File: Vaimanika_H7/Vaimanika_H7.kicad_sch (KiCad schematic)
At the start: 74 parts, among them CN1 WAFER-GH1.25-3PWB, J1 TYPE-C 16PIN 2MD, J2 Conn_01x09, J3 Conn_01x09, J4 +VLIPO, J5 GND, J6 Conn_01x09, J8 Conn_01x02, Q1 AO3400A, Q2 AO3401A, U1 TPS54302, U2 TPS54302, U3 USBLC6-2P6, U4 WAFER-GH1.25-4PWB, U5 WAFER-GH1.25-4PWB, U6 WAFER-GH1.25-4PWB, U7 WAFER-GH1.25-4PLB, U8 WAFER-GH1.25-4PLB, U9 WAFER-GH1.25-4PLB

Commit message: 05-05-2026
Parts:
- CN1: BOARD (none) -> POWER; LCSC (none) -> C3029378; LCSC Part C3029378 -> (none)
- FPC1, H1, H2, H3, H4, H5, H6, J1, J2, J3, J4, J5, J6, J8, U4, U5, U6, U7, U8, U9: BOARD (none) -> POWER

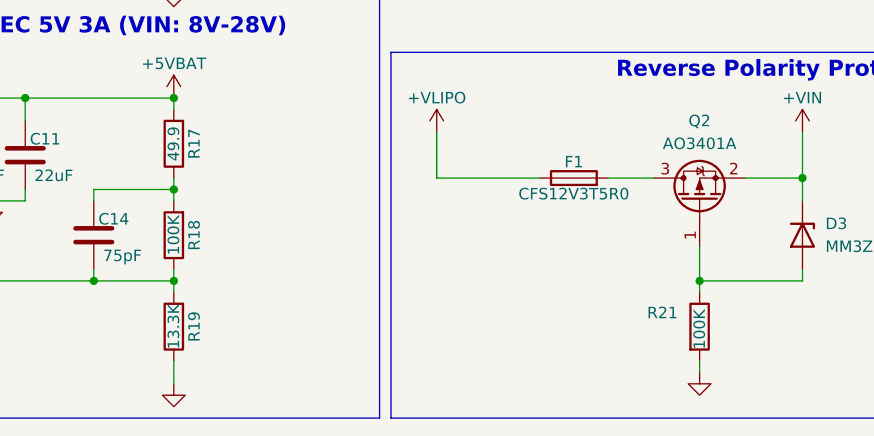
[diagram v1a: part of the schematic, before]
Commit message: 21-05-2026
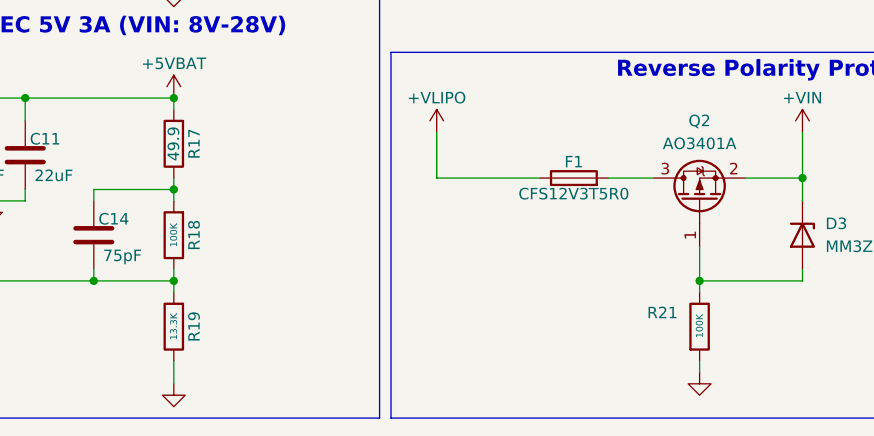
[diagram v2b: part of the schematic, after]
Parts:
- R17: LCSC C2909367 -> C87044
- R19: LCSC C2909367 -> C2974007
- R20: LCSC C60491 -> C2907233
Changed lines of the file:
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@@
 			)
 		)
-		(property "LCSC" "C60491"
+		(property "LCSC" "C2907233"
 			(at 163.83 62.23 90)
 			(effects
@@
 			(effects
 				(font
-					(size 1.27 1.27)
+					(size 0.762 0.762)
 				)
 			)
@@
 			)
 		)
-		(property "LCSC" "C2909367"
+		(property "LCSC" "C87044"
 			(at 147.32 160.02 90)
 			(effects
@@
 			(effects
 				(font
-					(size 1.27 1.27)
+					(size 0.762 0.762)
 				)
 			)
@@
 			)
 		)
-		(property "LCSC" "C2909367"
+		(property "LCSC" "C2974007"
 			(at 147.32 180.34 90)
 			(effects
@@
 		)
 		(property "Value" "100K"
-			(at 205.74 182.88 90)
+			(at 205.74 181.61 90)
 			(effects
 				(font
-					(size 1.27 1.27)
+					(size 0.762 0.762)
 				)
 				(justify left)

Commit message: 21-05-2026
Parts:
- J2, J3, J6: LCSC (none) -> C492408
- J8: LCSC (none) -> C492401
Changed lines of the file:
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@@
 			)
 		)
+		(property "LCSC" "C492408"
+			(at 204.47 68.58 0)
+			(effects
+				(font
+					(size 1.27 1.27)
+				)
+				(hide yes)
+			)
+		)
 		(pin "3"
 		)
@@
 			)
 		)
+		(property "LCSC" "C492408"
+			(at 228.6 71.12 0)
+			(effects
+				(font
+					(size 1.27 1.27)
+				)
+				(hide yes)
+			)
+		)
 		(pin "3"
 		)
@@
 			)
 		)
+		(property "LCSC" "C492401"
+			(at 254 33.02 0)
+			(effects
+				(font
+					(size 1.27 1.27)
+				)
+				(hide yes)
+			)
+		)
 		(pin "2"
 		)
@@
 			(at 204.47 44.45 0)
 			(effects
+				(font
+					(size 1.27 1.27)
+				)
+				(hide yes)
+			)
+		)
+		(property "LCSC" "C492408"
+			(at 204.47 44.45 0)
+			(effects

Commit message: 22-05-2026
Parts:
- J2, J3, J6: LCSC C492408 -> (none)
- J8: LCSC C492401 -> (none)
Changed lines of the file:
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@@
 			)
 		)
-		(property "LCSC" "C492408"
-			(at 204.47 68.58 0)
-			(effects
-				(font
-					(size 1.27 1.27)
-				)
-				(hide yes)
-			)
-		)
 		(pin "3"
 		)
@@
 			)
 		)
-		(property "LCSC" "C492408"
-			(at 228.6 71.12 0)
-			(effects
-				(font
-					(size 1.27 1.27)
-				)
-				(hide yes)
-			)
-		)
 		(pin "3"
 		)
@@
 			)
 		)
-		(property "LCSC" "C492401"
-			(at 254 33.02 0)
-			(effects
-				(font
-					(size 1.27 1.27)
-				)
-				(hide yes)
-			)
-		)
 		(pin "2"
 		)
@@
 			(at 204.47 44.45 0)
 			(effects
-				(font
-					(size 1.27 1.27)
-				)
-				(hide yes)
-			)
-		)
-		(property "LCSC" "C492408"
-			(at 204.47 44.45 0)
-			(effects
